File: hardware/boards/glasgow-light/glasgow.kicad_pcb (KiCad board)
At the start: 2 copper layers, 63.9 x 20.1 mm, 171 parts, among them J1 USB_C_USB2.0, J2 IDC-Header_2x5_P2.54mm, J3 IDC-Header_2x5_P2.54mm, U1 LM358_DFN, U10 SN74LVC1T45DCKR, U11 SN74LVC1T45DCKR, U12 INA180A2, U15 TPD3S014, U16 SN74LVC1T45DCKR, U17 SN74LVC1T45DCKR, U18 SN74LVC1T45DCKR, U19 PCA6408APW, U2 GD32VF103T, U31 TPS73101DBV, U36 TLV73312PQDRVR, U4 SN74LVC1T45DCKR, U5 ICE40UP5K-SG48ITR, U6 SN74LVC1T45DCKR, U8 TLV75533PDRVR, U9 SN74LVC1T45DCKR, Y1 8M

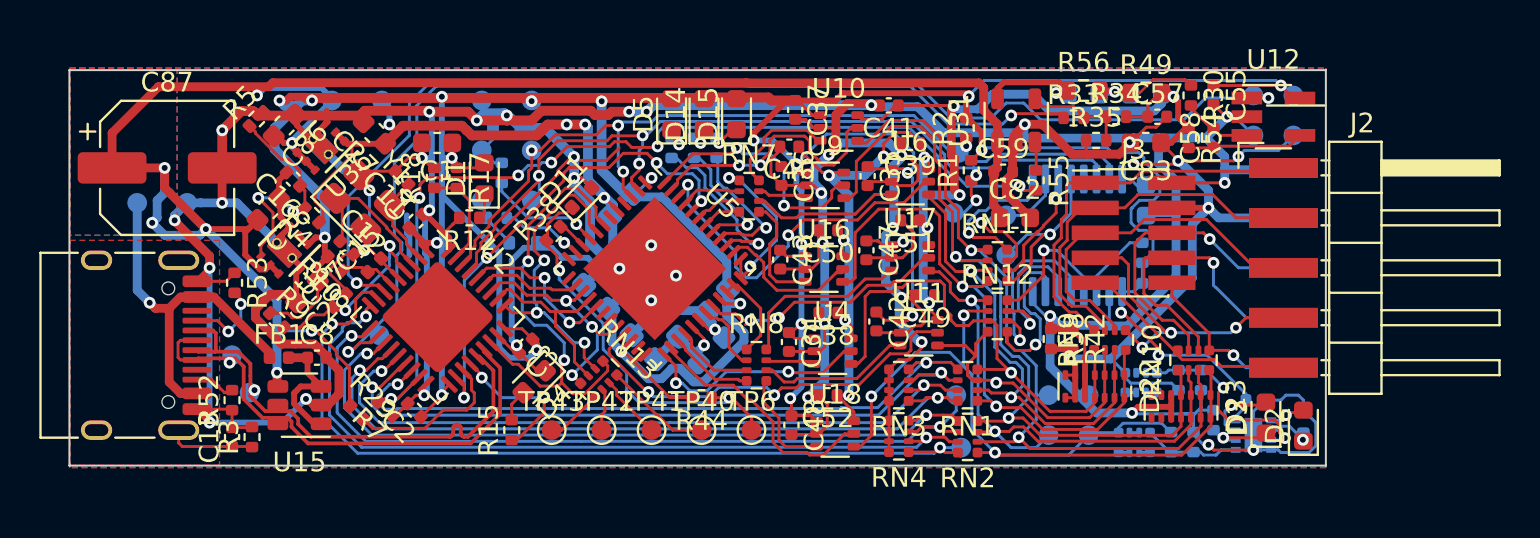
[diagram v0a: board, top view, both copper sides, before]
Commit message: make board another bit smaller -> outer size is metric
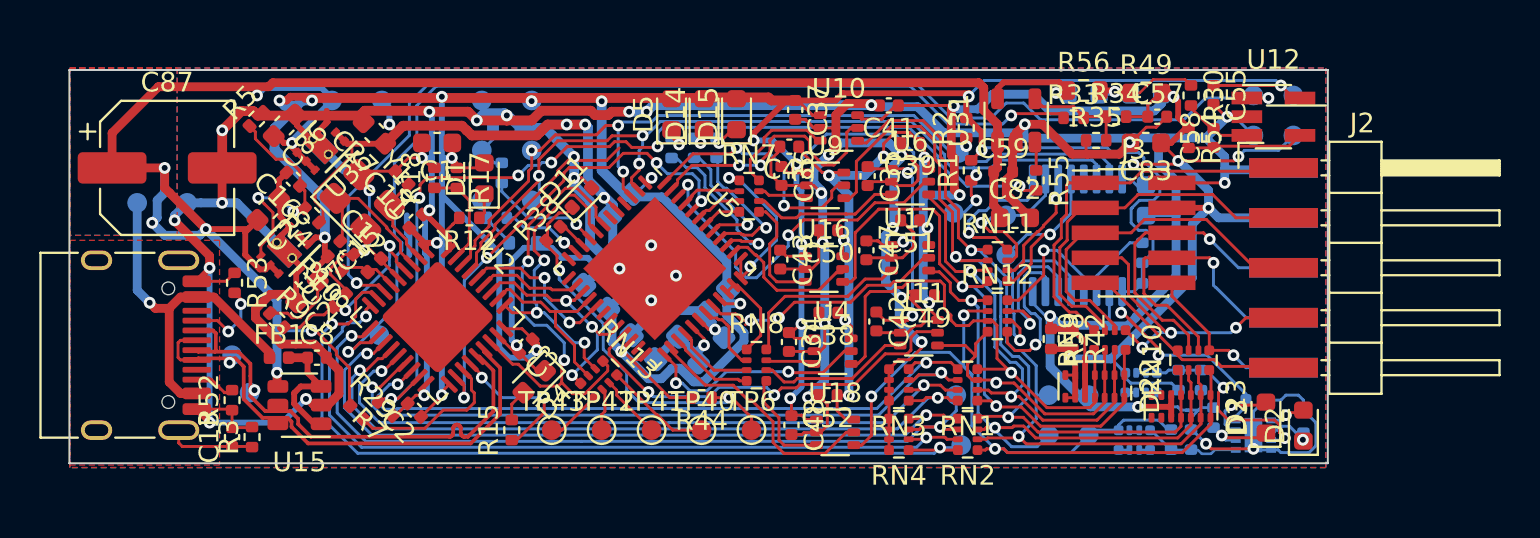
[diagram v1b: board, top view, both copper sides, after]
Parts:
- moved R14 0.18 mm to (167.3, 52.8)
- moved R19 0.13 mm to (168.4, 51.7)
- moved RN2 0.13 mm to (155.9, 52.5)
- moved R25 0.13 mm to (166.2, 52.8)
- moved TP29 0.13 mm to (155.6, 53.1)
- moved RN6 0.12 mm to (164.4, 52.8)
- moved RN4 0.10 mm to (152.4, 52.5)
- moved U18 0.08 mm to (149.2, 52.4)
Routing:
- net GND: track 389.8 -> 388.1 mm
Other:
- board size 63.9 x 20.1 mm -> 64 x 20 mm
